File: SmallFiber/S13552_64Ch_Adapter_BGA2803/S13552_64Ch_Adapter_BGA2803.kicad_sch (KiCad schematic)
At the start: 11 parts, among them J1 ERM6-30-01.5-L-DV-A-K-TR, J2 ERM6-30-01.5-L-DV-A-K-TR

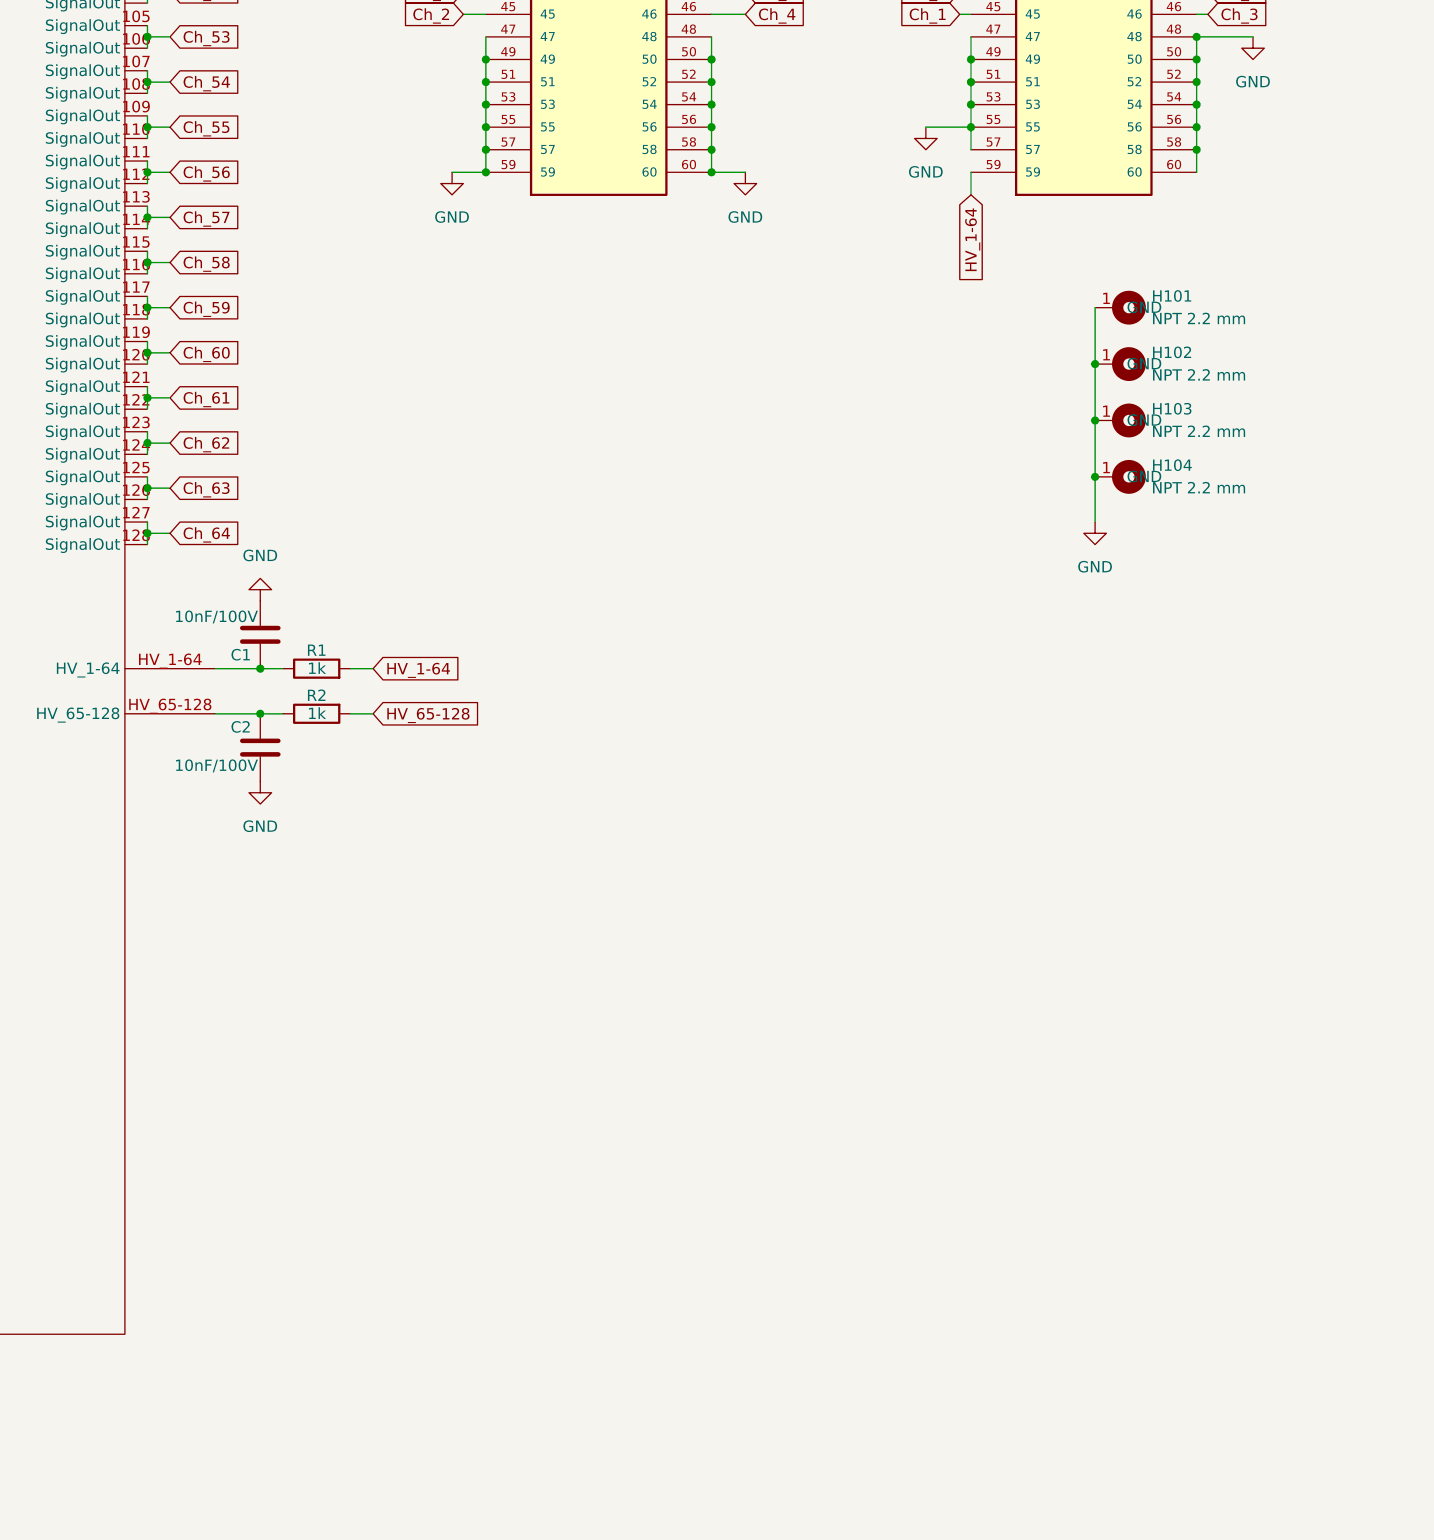
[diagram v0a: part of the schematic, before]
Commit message: .
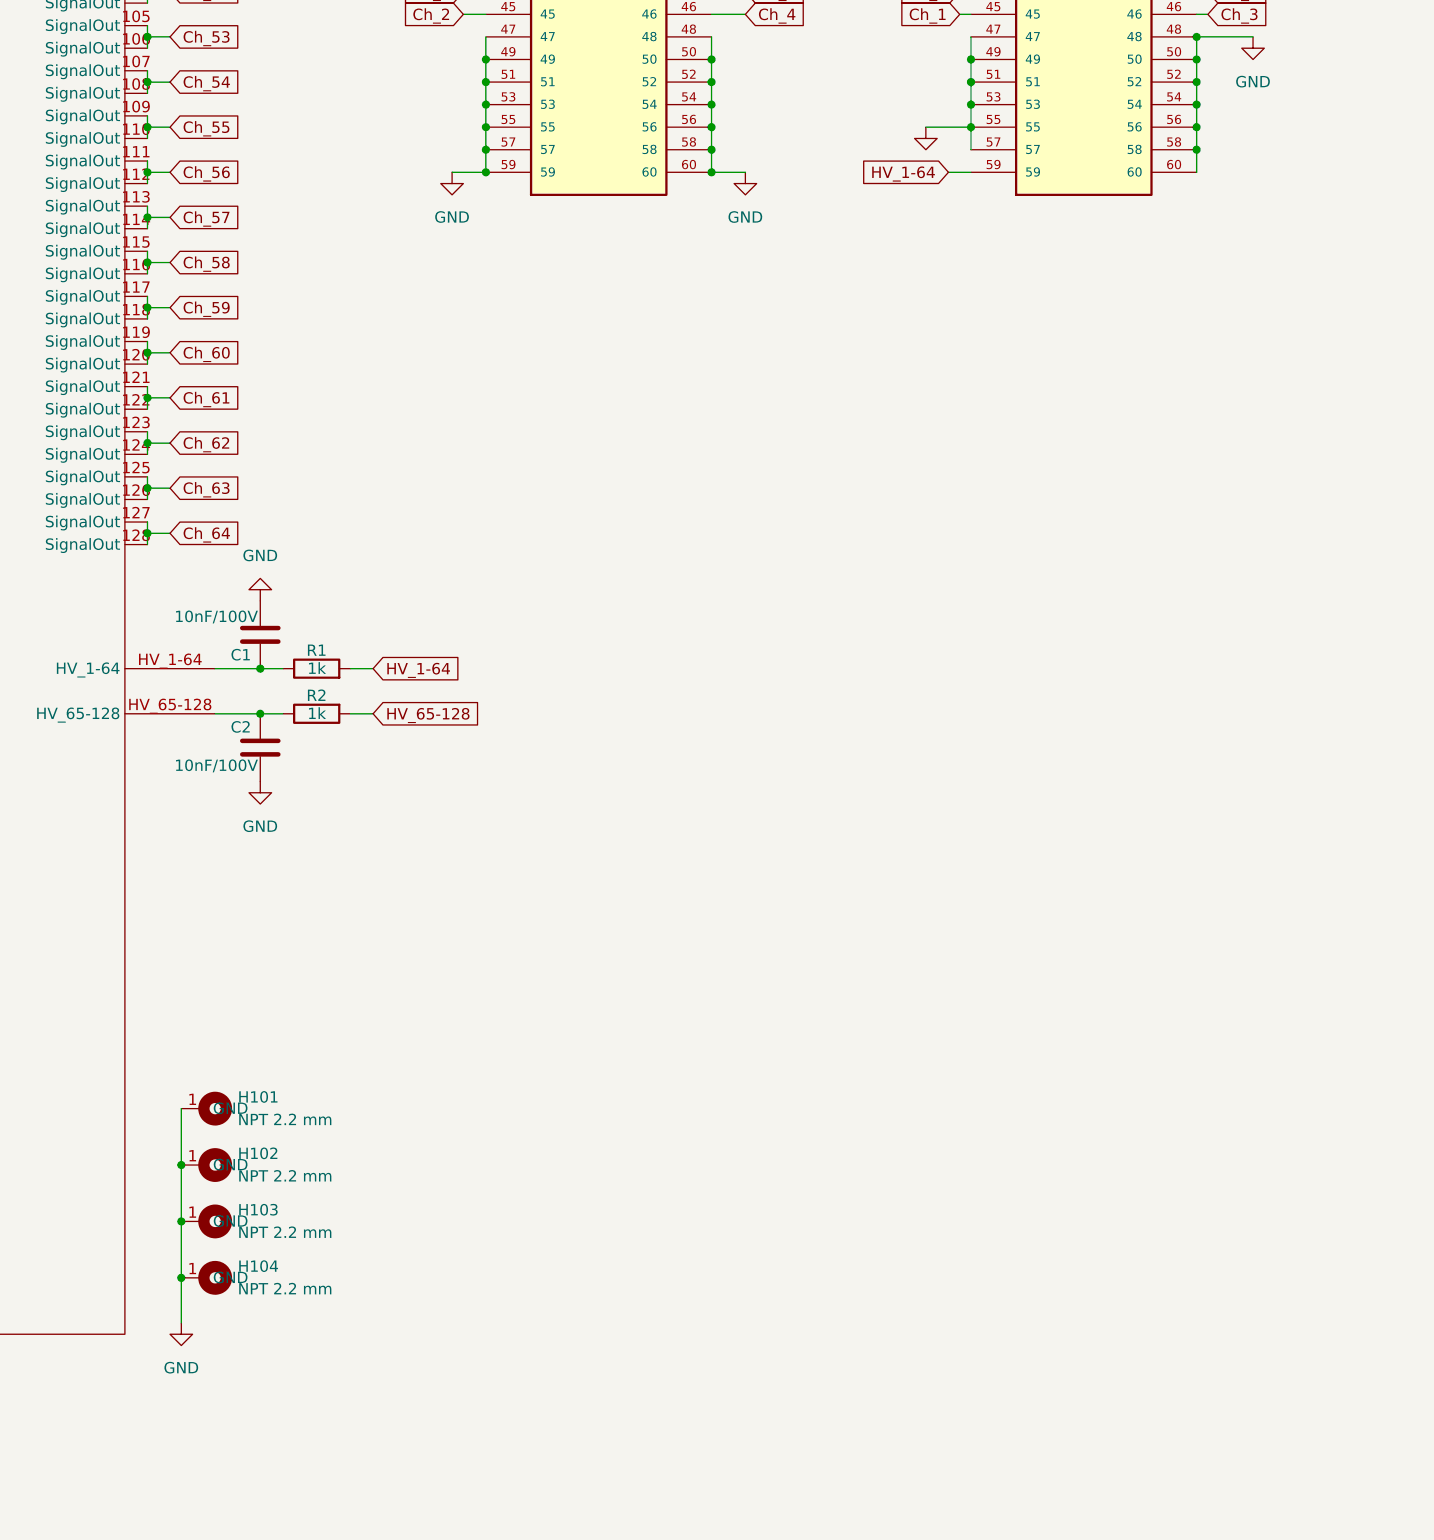
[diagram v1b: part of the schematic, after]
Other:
- moved on the sheet: H101, H102, H103, H104
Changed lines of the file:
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@@
 	)
 	(junction
-		(at 172.72 123.19)
+		(at 69.85 213.36)
 		(diameter 0)
 		(color 0 0 0 0)
@@
 	)
 	(junction
-		(at 172.72 135.89)
+		(at 69.85 226.06)
 		(diameter 0)
 		(color 0 0 0 0)
@@
 	)
 	(junction
-		(at 172.72 129.54)
+		(at 69.85 219.71)
 		(diameter 0)
 		(color 0 0 0 0)
@@
 	(wire
 		(pts
-			(xy 172.72 123.19) (xy 172.72 129.54)
+			(xy 69.85 213.36) (xy 69.85 219.71)
 		)
 		(stroke
@@
 	(wire
 		(pts
-			(xy 172.72 129.54) (xy 172.72 135.89)
+			(xy 69.85 219.71) (xy 69.85 226.06)
 		)
 		(stroke
@@
 	(wire
 		(pts
-			(xy 172.72 135.89) (xy 172.72 140.97)
+			(xy 69.85 226.06) (xy 69.85 231.14)
 		)
 		(stroke
@@
 	(wire
 		(pts
-			(xy 172.72 116.84) (xy 172.72 123.19)
+			(xy 69.85 207.01) (xy 69.85 213.36)
 		)
 		(stroke
@@
 	(wire
 		(pts
-			(xy 158.75 104.14) (xy 158.75 101.6)
-		)
-		(stroke
-			(width 0)
-			(type default)
-		)
-	)
-	(wire
-		(pts
 			(xy 33.02 119.38) (xy 33.02 120.65)
 		)
@@
 	(wire
 		(pts
+			(xy 156.21 101.6) (xy 158.75 101.6)
+		)
+		(stroke
+			(width 0)
+			(type default)
+		)
+	)
+	(wire
+		(pts
 			(xy 33.02 154.94) (xy 33.02 156.21)
 		)
@@
 	(global_label "HV_1-64"
 		(shape input)
-		(at 158.75 104.14 270)
+		(at 156.21 101.6 180)
 		(fields_autoplaced yes)
 		(effects
@@
 		)
 		(property "Intersheetrefs" "${INTERSHEET_REFS}"
-			(at 158.75 115.7128 90)
+			(at 144.6372 101.6 0)
 			(effects
 				(font
@@
 	(symbol
 		(lib_id "Mechanical:MountingHole")
-		(at 176.53 135.89 0)
+		(at 73.66 226.06 0)
 		(unit 1)
 		(exclude_from_sim yes)
@@
 		(fields_autoplaced yes)
 		(property "Reference" "H104"
-			(at 179.07 134.6199 0)
+			(at 76.2 224.7899 0)
 			(effects
 				(font
@@
 		)
 		(property "Value" "NPT 2.2 mm"
-			(at 179.07 137.1599 0)
+			(at 76.2 227.3299 0)
 			(effects
 				(font
@@
 		)
 		(property "Footprint" "MountingHole:MountingHole_2.2mm_M2"
-			(at 176.53 135.89 0)
+			(at 73.66 226.06 0)
 			(effects
 				(font
@@
 		)
 		(property "Datasheet" "~"
-			(at 176.53 135.89 0)
+			(at 73.66 226.06 0)
 			(effects
 				(font
@@
 		)
 		(property "Description" "Mounting Hole without connection"
-			(at 176.53 135.89 0)
+			(at 73.66 226.06 0)
 			(effects
 				(font
@@
 					(size 1.27 1.27)
 				)
+				(hide yes)
 			)
 		)
@@
 	(symbol
 		(lib_id "power:GND")
-		(at 172.72 140.97 0)
+		(at 69.85 231.14 0)
 		(unit 1)
 		(exclude_from_sim no)
@@
 		(fields_autoplaced yes)
 		(property "Reference" "#PWR09"
-			(at 172.72 147.32 0)
+			(at 69.85 237.49 0)
 			(effects
 				(font
@@
 		)
 		(property "Value" "GND"
-			(at 172.72 146.05 0)
+			(at 69.85 236.22 0)
 			(effects
 				(font
@@
 		)
 		(property "Footprint" ""
-			(at 172.72 140.97 0)
+			(at 69.85 231.14 0)
 			(effects
 				(font
@@
 		)
 		(property "Datasheet" ""
-			(at 172.72 140.97 0)
+			(at 69.85 231.14 0)
 			(effects
 				(font
@@
 		)
 		(property "Description" "Power symbol creates a global label with name \"GND\" , ground"
-			(at 172.72 140.97 0)
+			(at 69.85 231.14 0)
 			(effects
 				(font
@@
 		(lib_name "MountingHole_3")
 		(lib_id "Mechanical:MountingHole")
-		(at 176.53 129.54 0)
+		(at 73.66 219.71 0)
 		(unit 1)
 		(exclude_from_sim yes)
@@
 		(fields_autoplaced yes)
 		(property "Reference" "H103"
-			(at 179.07 128.2699 0)
+			(at 76.2 218.4399 0)
 			(effects
 				(font
@@
 		)
 		(property "Value" "NPT 2.2 mm"
-			(at 179.07 130.8099 0)
+			(at 76.2 220.9799 0)
 			(effects
 				(font
@@
 		)
 		(property "Footprint" "MountingHole:MountingHole_2.2mm_M2"
-			(at 176.53 129.54 0)
+			(at 73.66 219.71 0)
 			(effects
 				(font
@@
 		)
 		(property "Datasheet" "~"
-			(at 176.53 129.54 0)
+			(at 73.66 219.71 0)
 			(effects
 				(font
@@
 		)
 		(property "Description" "Mounting Hole without connection"
-			(at 176.53 129.54 0)
+			(at 73.66 219.71 0)
 			(effects
 				(font
@@
 		(lib_name "MountingHole_2")
 		(lib_id "Mechanical:MountingHole")
-		(at 176.53 123.19 0)
+		(at 73.66 213.36 0)
 		(unit 1)
 		(exclude_from_sim yes)
@@
 		(fields_autoplaced yes)
 		(property "Reference" "H102"
-			(at 179.07 121.9199 0)
+			(at 76.2 212.0899 0)
 			(effects
 				(font
@@
 		)
 		(property "Value" "NPT 2.2 mm"
-			(at 179.07 124.4599 0)
+			(at 76.2 214.6299 0)
 			(effects
 				(font
@@
 		)
 		(property "Footprint" "MountingHole:MountingHole_2.2mm_M2"
-			(at 176.53 123.19 0)
+			(at 73.66 213.36 0)
 			(effects
 				(font
@@
 		)
 		(property "Datasheet" "~"
-			(at 176.53 123.19 0)
+			(at 73.66 213.36 0)
 			(effects
 				(font
@@
 		)
 		(property "Description" "Mounting Hole without connection"
-			(at 176.53 123.19 0)
+			(at 73.66 213.36 0)
 			(effects
 				(font
@@
 		(lib_name "MountingHole_1")
 		(lib_id "Mechanical:MountingHole")
-		(at 176.53 116.84 0)
+		(at 73.66 207.01 0)
 		(unit 1)
 		(exclude_from_sim yes)
@@
 		(fields_autoplaced yes)
 		(property "Reference" "H101"
-			(at 179.07 115.5699 0)
+			(at 76.2 205.7399 0)
 			(effects
 				(font
@@
 		)
 		(property "Value" "NPT 2.2 mm"
-			(at 179.07 118.1099 0)
+			(at 76.2 208.2799 0)
 			(effects
 				(font
@@
 		)
 		(property "Footprint" "MountingHole:MountingHole_2.2mm_M2"
-			(at 176.53 116.84 0)
+			(at 73.66 207.01 0)
 			(effects
 				(font
@@
 		)
 		(property "Datasheet" "~"
-			(at 176.53 116.84 0)
+			(at 73.66 207.01 0)
 			(effects
 				(font
@@
 		)
 		(property "Description" "Mounting Hole without connection"
-			(at 176.53 116.84 0)
+			(at 73.66 207.01 0)
 			(effects
 				(font
